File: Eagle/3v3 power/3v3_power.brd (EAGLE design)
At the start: 61.9 x 74.9 mm, 32 parts, among them IC1 7805TV, IC2 LD117AS12TR, IC4 7812TV

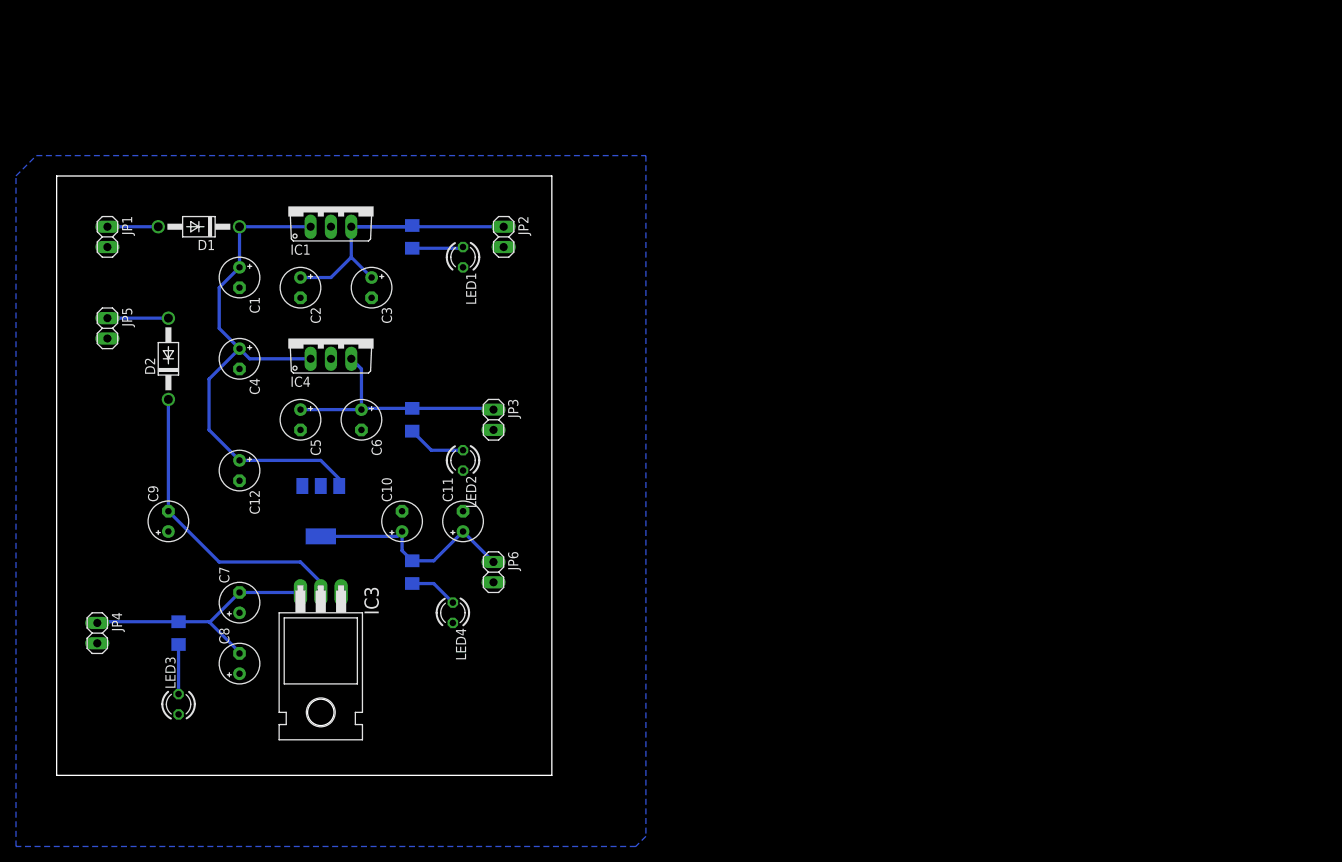
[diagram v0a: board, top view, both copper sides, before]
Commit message: schematics
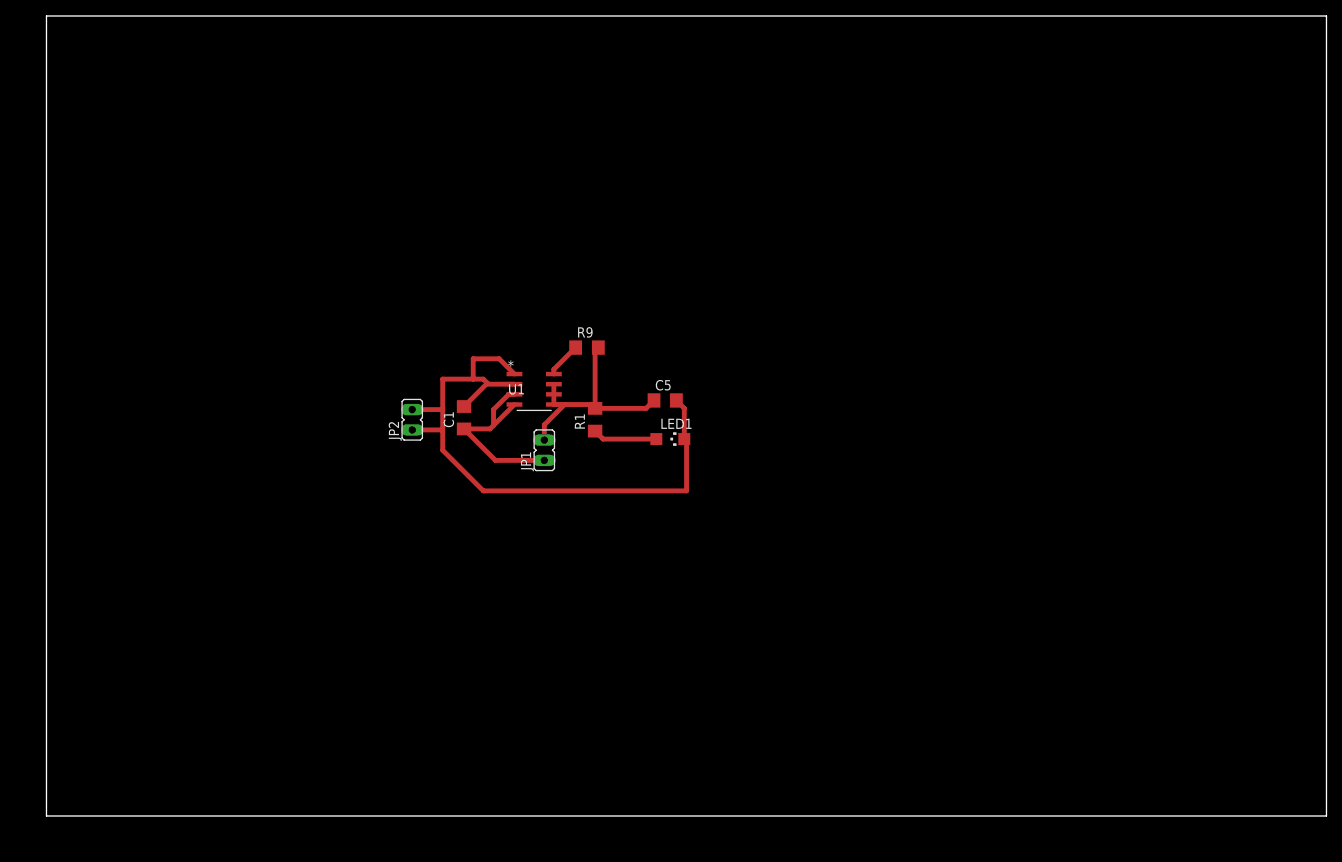
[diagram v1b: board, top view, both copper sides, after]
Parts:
- removed C10, C11, C12, C2, C3, C4, C6, C7, C8, C9: (no value), rcl:E2,5-5
- removed D1, D2: 1N4004, diode:DO41-10
- removed IC1: 7805TV, linear:TO220V
- removed IC2: LD117AS12TR, v-reg:SOT223
- removed IC3: (no value), linear:TO220H
- removed IC4: 7812TV, linear:TO220V
- removed JP3, JP4, JP5, JP6: (no value), pinhead:1X02
- removed LED2, LED3, LED4: (no value), led:LED3MM
- removed R5, R6, R7: (no value), rcl:R1206
- added R9: (no value), rcl:R1206
- added U1: TPS7333QD, TPS7333:D8
- C1, C5: device rcl:E2,5-5 -> rcl:C1206
- JP1, JP2: device pinhead:1X02 -> jumper:JP1
- LED1: value (none) -> TXLED; device led:LED3MM -> led:CHIPLED_1206
- moved JP1 60.8 mm to (62.2, 45.7), turned to 0 degrees
- moved C5 45.7 mm to (77.3, 51.9), turned to 0 degrees
- moved LED1 34.5 mm to (78.0, 47.1)
- moved C1 33.1 mm to (52.2, 49.8), turned to 90 degrees
- moved R1 29.8 mm to (68.6, 49.5), flipped to the top
- moved JP2 25.6 mm to (45.7, 49.5), turned to 0 degrees
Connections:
- removed net N$1: D1.A, JP1.1
- removed net N$10: C7.-, C8.-, IC3.3, JP4.1, R5.2
- removed net N$11: C1.+, C12.+, C4.+, D1.C, IC1.1, IC2.3, IC4.1
- removed net N$12: C10.+, C11.+, IC2.4, JP6.1, R1.2
- removed net N$6: C2.+, C3.+, IC1.3, JP2.1, R6.2
- removed net N$7: C5.+, C6.+, IC4.3, JP3.1, R7.2
- removed net N$8: LED2.A, R7.1
- removed net N$9: LED3.K, R5.1
- net GND: now also C1.2, C5.2, JP2.1, LED1.C, U1.1, U1.2; no longer C1.-, C10.-, C11.-, C12.-, C2.-, C3.-, C4.-, C5.-, C6.-, C7.+, C8.+, C9.+, IC1.2, IC2.1, IC3.1, IC4.2, JP1.2, JP3.2, JP4.2, JP5.2, JP6.2, LED1.K, LED2.K, LED3.A, LED4.K
- net N$2: now also C1.1, JP1.1, U1.3, U1.4; no longer C9.-, D2.C, IC3.2
- net N$3: now also C5.1, JP1.2, R1.2, R9.2, U1.5, U1.6, U1.7; no longer D2.A, JP5.1
- net N$4: now also R9.1, U1.8; no longer LED4.A, R1.1
- net N$5: now also R1.1; no longer R6.1
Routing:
- net GND: track 0.00 -> 82.6 mm
- net N$11: track 67.1 -> 0.00 mm
- net N$6: track 41.5 -> 0.00 mm
- net N$10: track 32.5 -> 0.00 mm
- net N$7: track 31.1 -> 0.00 mm
- net N$12: track 27.9 -> 0.00 mm
- net N$3: track 7.62 -> 28.9 mm
- net N$2: track 38.0 -> 24.6 mm
- net N$8: track 7.34 -> 0.00 mm
- net N$1: track 6.35 -> 0.00 mm
- net N$9: track 6.20 -> 0.00 mm
- net N$5: track 6.41 -> 8.06 mm
- net N$4: track 6.07 -> 4.43 mm
- removed copper zone on layer 16, net GND
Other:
- board size 61.9 x 74.9 mm -> 160 x 100 mm
